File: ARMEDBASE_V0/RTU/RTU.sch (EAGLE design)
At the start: 10 parts, among them Q2 2N3904

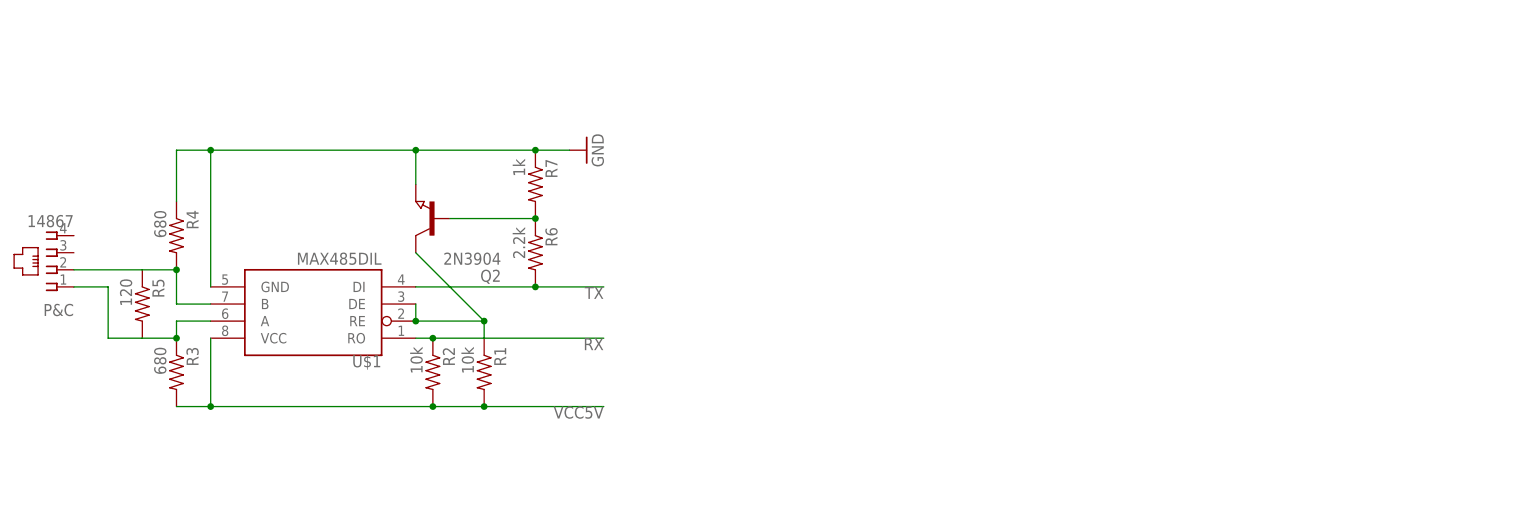
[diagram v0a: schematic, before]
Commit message: rtu
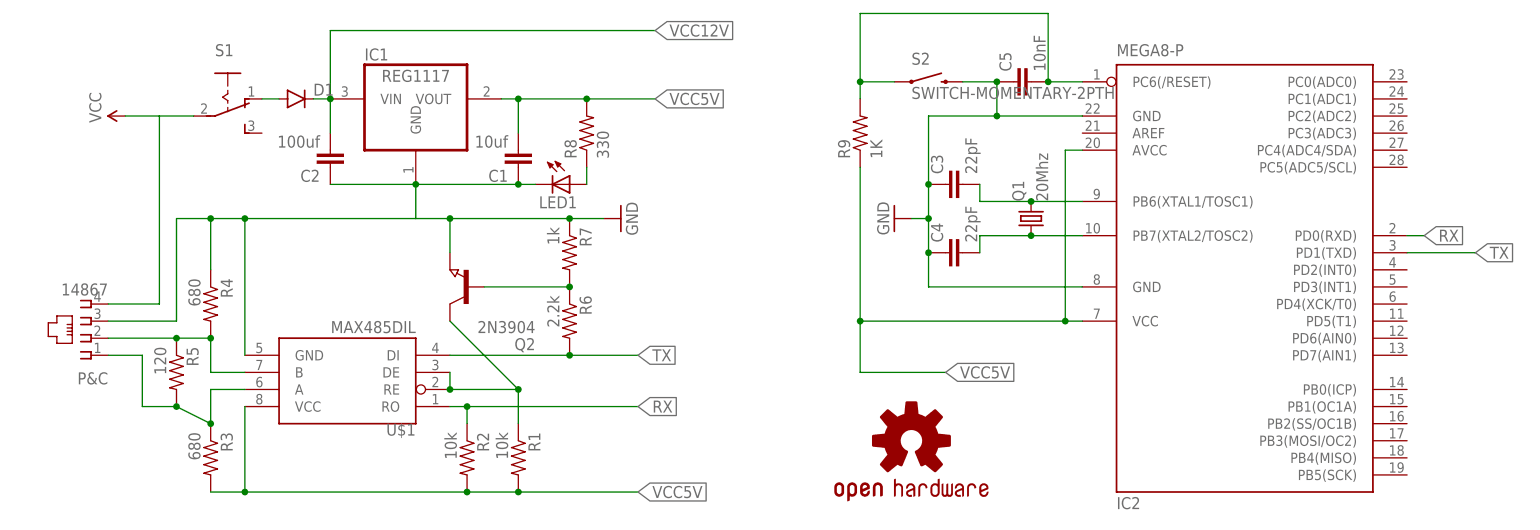
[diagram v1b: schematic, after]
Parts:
- added C1: 10uf, SparkFun-Capacitors:CAP0805
- added C2: 100uf, SparkFun-Capacitors:CAP0805
- added C3, C4: 22pF, SparkFun-Capacitors:CAP0805
- added C5: 10nF, SparkFun-Capacitors:CAP0805
- added D1: (no value), SparkFun-DiscreteSemi:DIODESMA
- added IC1: REG1117, burr-brown:REG1117
- added IC2: MEGA8-P, atmel:MEGA8-P
- added LED1: (no value), led:LEDCHIP-LED0805
- added LOGO1: OSHW-LOGOL, SparkFun-Aesthetics:OSHW-LOGOL
- added Q1: 20Mhz, crystal:CRYSTALSM49
- added R8: 330, SparkFun-Passives:RESISTOR0805-RES
- added R9: 1K, SparkFun-Passives:RESISTOR0805-RES
- added S1: (no value), switch:255SB
- added S2: SWITCH-MOMENTARY-2PTH, SparkFun-Electromechanical:SWITCH-MOMENTARY-2PTH
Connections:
- new net N$11: LED1.A, R8.1
- new net N$13: D1.A, S1.O
- new net N$21: C3.2, IC2.PB6(XTAL1/TOSC1), Q1.2
- new net N$23: C4.2, IC2.PB7(XTAL2/TOSC2), Q1.1
- new net N$24: C5.2, IC2.PC6(/RESET), R9.2, S2.1
- new net VCC: P&C.4, S1.P
- new net VCC12V: C2.2, D1.C, IC1.VIN
- net GND: now also C1.1, C2.1, C3.1, C4.1, C5.1, IC1.GND, IC2.GND, IC2.GND@1, LED1.C, P&C.3, S2.2
- net RX: now also IC2.PD0(RXD)
- net TX: now also IC2.PD1(TXD)
- net VCC5V: now also C1.2, IC1.VOUT, IC2.AVCC, IC2.VCC@1, R8.2, R9.1
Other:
- moved on the sheet: P&C, Q2, R1, R2, R3, R4, R5, R6, R7, U$1
